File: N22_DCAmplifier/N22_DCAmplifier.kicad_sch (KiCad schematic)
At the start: 81 parts

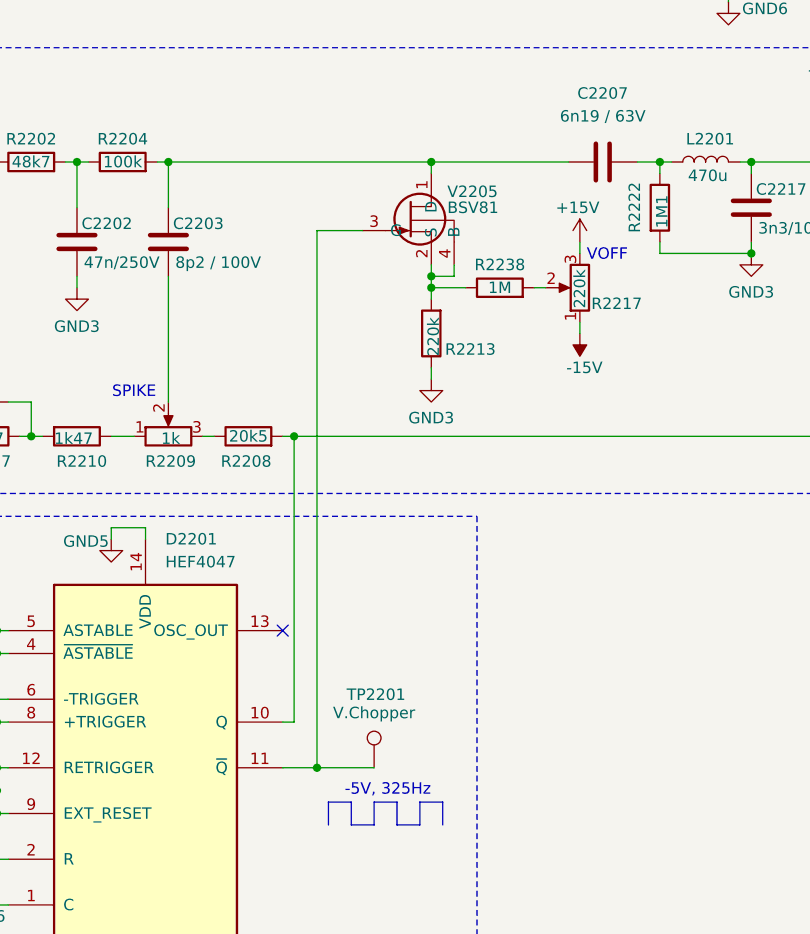
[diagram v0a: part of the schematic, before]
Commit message: Small updates, N25 also
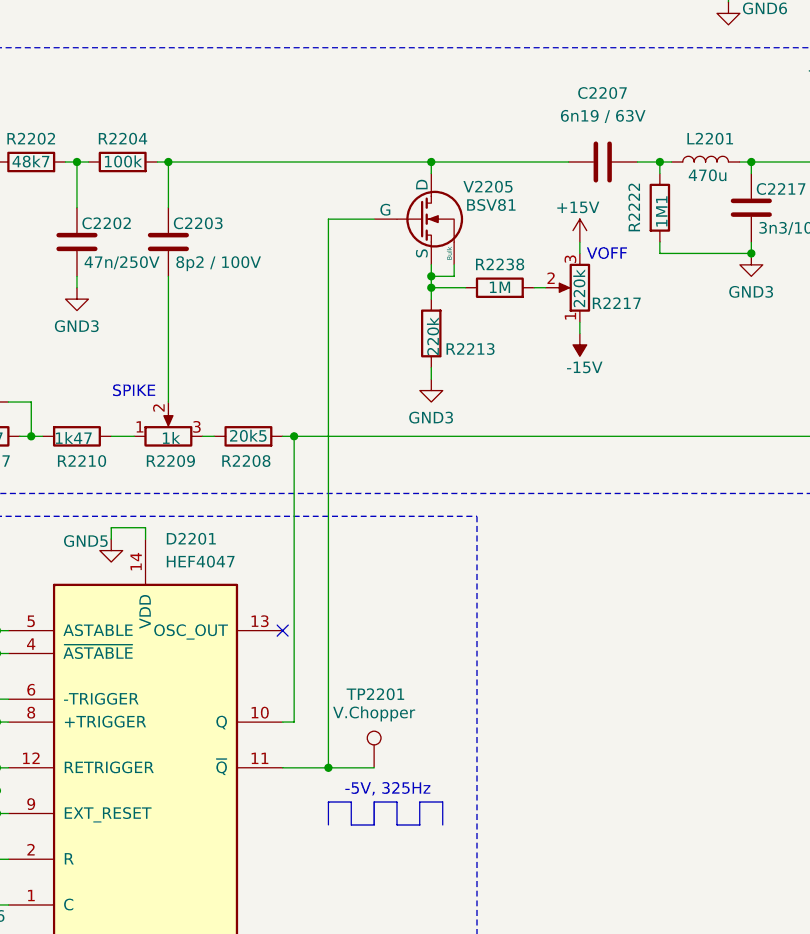
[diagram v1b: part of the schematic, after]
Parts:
- removed V2205: BSV81, Package_TO_SOT_THT:TO-72-4, symbol PM2528:BVS81
- added V2205: BSV81, Package_TO_SOT_THT:TO-72-4, symbol Simulation_SPICE:NMOS_Substrate
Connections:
- net at C2203.2, C2207.1, R2204.2: now also V2205.1 (D)
- net at D2201.11 (~{Q}), TP2201.1: now also V2205.2 (G)
- net at R2213.2, R2238.1: now also V2205.3 (S), V2205.4 (Bulk)
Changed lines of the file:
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@@
 	)
 	(junction
-		(at 127 246.38)
-		(diameter 0)
-		(color 0 0 0 0)
-	)
-	(junction
 		(at 372.11 215.9)
 		(diameter 0)
@@
 	)
 	(junction
+		(at 139.7 179.07)
+		(diameter 0)
+		(color 0 0 0 0)
+	)
+	(junction
 		(at 85.09 209.55)
 		(diameter 0)
@@
 	)
 	(junction
-		(at 139.7 179.07)
-		(diameter 0)
-		(color 0 0 0 0)
-	)
-	(junction
 		(at 142.24 71.12)
 		(diameter 0)
@@
 	)
 	(junction
+		(at 128.27 246.38)
+		(diameter 0)
+		(color 0 0 0 0)
+	)
+	(junction
 		(at 172.72 151.13)
 		(diameter 0)
@@
 	(wire
 		(pts
-			(xy 127 186.69) (xy 127 246.38)
+			(xy 128.27 185.42) (xy 128.27 246.38)
 		)
 		(stroke
@@
 	(wire
 		(pts
+			(xy 139.7 179.07) (xy 139.7 180.34)
+		)
+		(stroke
+			(width 0)
+			(type default)
+		)
+	)
+	(wire
+		(pts
 			(xy 90.17 261.62) (xy 92.71 261.62)
 		)
@@
 	(wire
 		(pts
-			(xy 123.19 246.38) (xy 127 246.38)
+			(xy 123.19 246.38) (xy 128.27 246.38)
 		)
 		(stroke
@@
 	(wire
 		(pts
+			(xy 128.27 246.38) (xy 133.35 246.38)
+		)
+		(stroke
+			(width 0)
+			(type default)
+		)
+	)
+	(wire
+		(pts
 			(xy 93.98 27.94) (xy 93.98 29.21)
 		)
@@
 	(wire
 		(pts
-			(xy 139.7 180.34) (xy 139.7 179.07)
-		)
-		(stroke
-			(width 0)
-			(type default)
-		)
-	)
-	(wire
-		(pts
 			(xy 388.62 215.9) (xy 388.62 217.17)
 		)
@@
 	(wire
 		(pts
+			(xy 139.7 179.07) (xy 154.94 179.07)
+		)
+		(stroke
+			(width 0)
+			(type default)
+		)
+	)
+	(wire
+		(pts
 			(xy 166.37 92.71) (xy 166.37 93.98)
 		)
@@
 	(wire
 		(pts
-			(xy 139.7 179.07) (xy 154.94 179.07)
-		)
-		(stroke
-			(width 0)
-			(type default)
-		)
-	)
-	(wire
-		(pts
 			(xy 350.52 44.45) (xy 350.52 45.72)
 		)
@@
 	(wire
 		(pts
-			(xy 127 246.38) (xy 133.35 246.38)
-		)
-		(stroke
-			(width 0)
-			(type default)
-		)
-	)
-	(wire
-		(pts
 			(xy 95.25 209.55) (xy 93.98 209.55)
 		)
@@
 	(wire
 		(pts
-			(xy 127 186.69) (xy 132.08 186.69)
+			(xy 128.27 185.42) (xy 133.35 185.42)
 		)
 		(stroke
@@
 	)
 	(symbol
+		(lib_id "Simulation_SPICE:NMOS_Substrate")
+		(at 137.16 185.42 0)
+		(unit 1)
+		(exclude_from_sim no)
+		(in_bom yes)
+		(on_board yes)
+		(dnp no)
+		(property "Reference" "V2205"
+			(at 143.256 181.864 0)
+			(effects
+				(font
+					(size 1.27 1.27)
+				)
+				(justify left)
+			)
+		)
+		(property "Value" "BSV81"
+			(at 143.51 183.896 0)
+			(effects
+				(font
+					(size 1.27 1.27)
+				)
+				(justify left)
+			)
+		)
+		(property "Footprint" "Package_TO_SOT_THT:TO-72-4"
+			(at 167.005 185.42 0)
+			(effects
+				(font
+					(size 1.27 1.27)
+				)
+				(hide yes)
+			)
+		)
+		(property "Datasheet" "https://ngspice.sourceforge.io/docs/ngspice-html-manual/manual.xhtml#cha_MOSFETs"
+			(at 137.16 204.47 0)
+			(effects
+				(font
+					(size 1.27 1.27)
+				)
+				(hide yes)
+			)
+		)
+		(property "Description" "N-channel MOSFET symbol with substrate (bulk) pin"
+			(at 137.16 185.42 0)
+			(effects
+				(font
+					(size 1.27 1.27)
+				)
+				(hide yes)
+			)
+		)
+		(property "Sim.Device" "NMOS"
+			(at 137.16 201.93 0)
+			(effects
+				(font
+					(size 1.27 1.27)
+				)
+				(hide yes)
+			)
+		)
+		(property "Sim.Type" "MOS1"
+			(at 137.16 200.025 0)
+			(effects
+				(font
+					(size 1.27 1.27)
+				)
+				(hide yes)
+			)
+		)
+		(property "Sim.Pins" "1=D 2=G 3=S 4=B"
+			(at 137.16 198.12 0)
+			(effects
+				(font
+					(size 1.27 1.27)
+				)
+				(hide yes)
+			)
+		)
+		(pin "3"
+		)
+		(pin "1"
+		)
+		(pin "2"
+		)
+		(pin "4"
+		)
+		(instances
+			(project ""
+				(path "/2ba4ca6b-4aec-411c-9da4-218d92fedde9"
+					(reference "V2205")
+					(unit 1)
+				)
+			)
+		)
+	)
+	(symbol
 		(lib_id "Diode:BAW75")
 		(at 72.39 29.21 180)
@@
 					(unit 1)
 				)
-			)
-		)
-	)
-	(symbol
-		(lib_id "PM2528:BVS81")
-		(at 138.43 185.42 0)
-		(unit 1)
-		(exclude_from_sim no)
-		(in_bom yes)
-		(on_board yes)
-		(dnp no)
-		(property "Reference" "V2205"
-			(at 141.478 182.372 0)
-			(effects
-				(font
-					(size 1.27 1.27)
-				)
-				(justify left)
-			)
-		)
-		(property "Value" "BSV81"
-			(at 141.478 184.15 0)
-			(effects
-				(font
-					(size 1.27 1.27)
-				)
-				(justify left)
-			)
-		)
-		(property "Footprint" "Package_TO_SOT_THT:TO-72-4"
-			(at 138.43 185.42 0)
-			(effects
-				(font
-					(size 1.27 1.27)
-				)
-				(hide yes)
-			)
-		)
-		(property "Datasheet" ""
-			(at 138.43 185.42 0)
-			(effects
-				(font
-					(size 1.27 1.27)
-				)
-				(hide yes)
-			)
-		)
-		(property "Description" ""
-			(at 138.43 185.42 0)
-			(effects
-				(font
-					(size 1.27 1.27)
-				)
-				(hide yes)
-			)
-		)
-		(pin "2"
-		)
-		(pin "4"
-		)
-		(pin "3"
-		)
-		(pin "1"
-		)
-		(instances
-			(project ""
-				(path "/2ba4ca6b-4aec-411c-9da4-218d92fedde9"
-					(reference "V2205")
-					(unit 1)
-				)
